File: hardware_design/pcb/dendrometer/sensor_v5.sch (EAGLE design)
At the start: 27 parts, among them J1 AVR_SPI_PRG_6PTH, Q2 MOSFET-P, U1 ATMEGA328P, U2 LM4040A20IDBZT

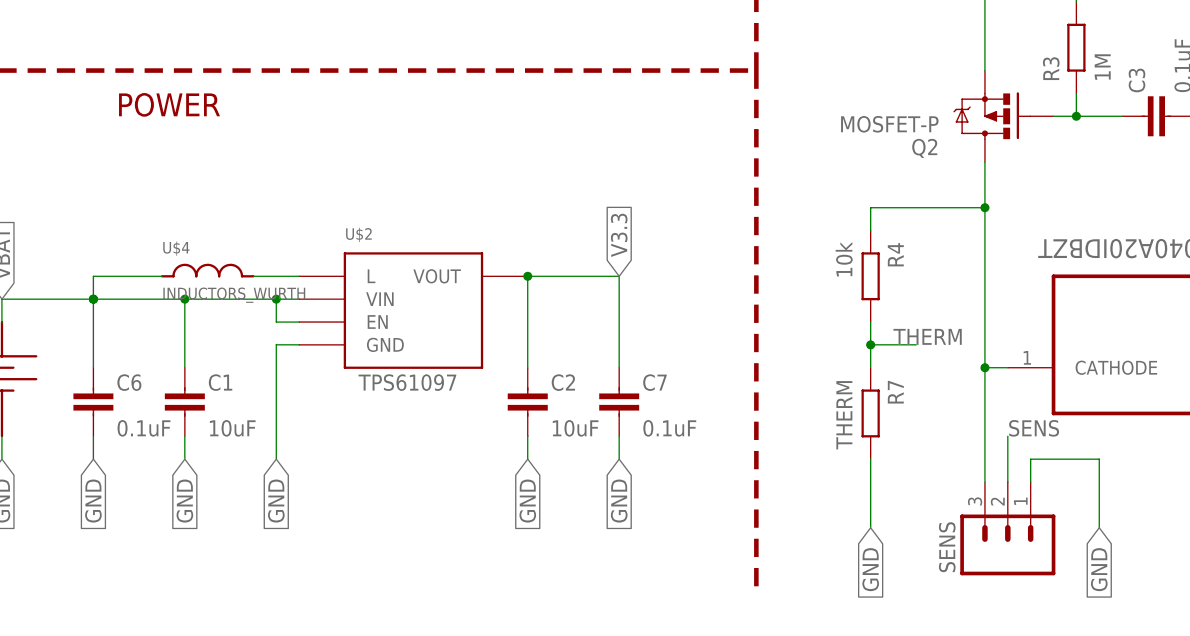
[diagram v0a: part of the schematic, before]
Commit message: cleanup..
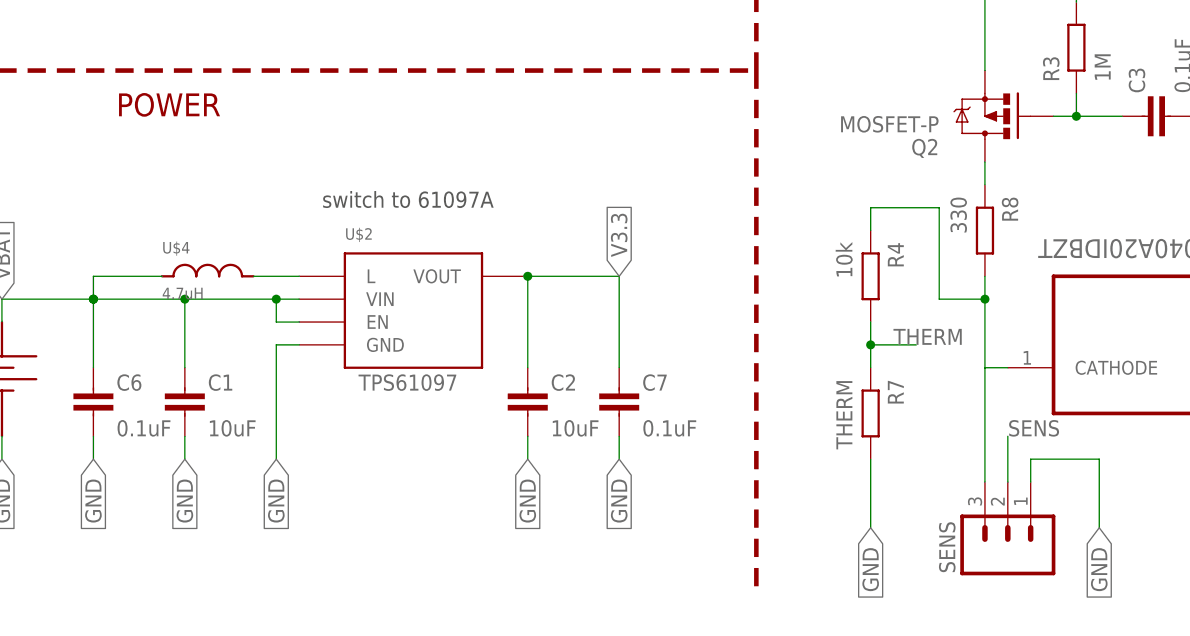
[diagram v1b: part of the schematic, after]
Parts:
- added R8: 330, passives-7351:RESISTOR0603-N
- U$4: value INDUCTORS_WURTH -> 4.7uH
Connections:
- new net S_EN: Q2.D, R8.P$1
- net V_REF: now also R8.P$2; no longer Q2.D
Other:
- note added: "switch to 61097A"
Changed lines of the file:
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@@
 <?xml version="1.0" encoding="utf-8"?>
 <!DOCTYPE eagle SYSTEM "eagle.dtd">
-<eagle version="7.2.0">
+<eagle version="7.6.0">
 <drawing>
 <settings>
@@
 <setting verticaltext="up"/>
 </settings>
-<grid distance="0.1" unitdist="inch" unit="inch" style="lines" multiple="1" display="no" altdistance="0.01" altunitdist="inch" altunit="inch"/>
+<grid distance="0.1" unitdist="inch" unit="inch" style="lines" multiple="1" display="yes" altdistance="0.01" altunitdist="inch" altunit="inch"/>
 <layers>
 <layer number="1" name="Top" color="4" fill="1" visible="no" active="no"/>
+<layer number="2" name="Route2" color="1" fill="3" visible="no" active="no"/>
+<layer number="3" name="Route3" color="4" fill="3" visible="no" active="no"/>
+<layer number="4" name="Route4" color="1" fill="4" visible="no" active="no"/>
+<layer number="5" name="Route5" color="4" fill="4" visible="no" active="no"/>
+<layer number="6" name="Route6" color="1" fill="8" visible="no" active="no"/>
+<layer number="7" name="Route7" color="4" fill="8" visible="no" active="no"/>
+<layer number="8" name="Route8" color="1" fill="2" visible="no" active="no"/>
+<layer number="9" name="Route9" color="4" fill="2" visible="no" active="no"/>
+<layer number="10" name="Route10" color="1" fill="7" visible="no" active="no"/>
+<layer number="11" name="Route11" color="4" fill="7" visible="no" active="no"/>
+<layer number="12" name="Route12" color="1" fill="5" visible="no" active="no"/>
+<layer number="13" name="Route13" color="4" fill="5" visible="no" active="no"/>
+<layer number="14" name="Route14" color="1" fill="6" visible="no" active="no"/>
+<layer number="15" name="Route15" color="4" fill="6" visible="no" active="no"/>
 <layer number="16" name="Bottom" color="1" fill="1" visible="no" active="no"/>
 <layer number="17" name="Pads" color="2" fill="1" visible="no" active="no"/>
@@
 <part name="U$5" library="LowPowerLab" deviceset="RFM69" device=""/>
 <part name="U$2" library="_my-parts" deviceset="TPS61097-33" device=""/>
-<part name="U$4" library="_my-parts" deviceset="INDUCTORS" device="_WURTH"/>
+<part name="U$4" library="_my-parts" deviceset="INDUCTORS" device="_WURTH" value="4.7uH"/>
 <part name="C1" library="passives-7351" deviceset="CAPACITOR" device="0805-N" value="10uF"/>
 <part name="C2" library="passives-7351" deviceset="CAPACITOR" device="0805-N" value="10uF"/>
@@
 <part name="R4" library="passives-7351" deviceset="RESISTOR" device="0603-N" value="10k"/>
 <part name="FRAME1" library="SparkFun-Aesthetics" deviceset="FRAME-A4L" device=""/>
+<part name="R8" library="passives-7351" deviceset="RESISTOR" device="0603-N" value="330"/>
 </parts>
 <sheets>
@@
 <text x="218.44" y="93.98" size="1.778" layer="94">ADC</text>
 <text x="129.54" y="93.98" size="1.778" layer="94">V_REF</text>
+<text x="50.8" y="48.26" size="1.778" layer="97">switch to 61097A</text>
 </plain>
 <instances>
@@
 <instance part="R4" gate="G$1" x="111.76" y="40.64" rot="R270"/>
 <instance part="FRAME1" gate="G$1" x="3.81" y="3.81"/>
+<instance part="R8" gate="G$1" x="124.46" y="45.72" rot="R270"/>
 </instances>
 <busses>
@@
 </segment>
 </net>
-<net name="V_REF" class="0">
-<segment>
-<pinref part="SENS" gate="J$1" pin="3"/>
-<wire x1="124.46" y1="17.78" x2="124.46" y2="30.48" width="0.1524" layer="91"/>
-<pinref part="U2" gate="A" pin="CATHODE"/>
-<wire x1="127" y1="30.48" x2="124.46" y2="30.48" width="0.1524" layer="91"/>
+<net name="S_EN" class="0">
+<segment>
+<pinref part="R8" gate="G$1" pin="P$1"/>
 <pinref part="Q2" gate="G$1" pin="D"/>
-<wire x1="124.46" y1="30.48" x2="124.46" y2="48.26" width="0.1524" layer="91"/>
-<junction x="124.46" y="30.48"/>
-<wire x1="124.46" y1="48.26" x2="124.46" y2="53.34" width="0.1524" layer="91"/>
-<pinref part="R4" gate="G$1" pin="P$1"/>
-<wire x1="111.76" y1="45.72" x2="111.76" y2="48.26" width="0.1524" layer="91"/>
-<wire x1="111.76" y1="48.26" x2="124.46" y2="48.26" width="0.1524" layer="91"/>
-<junction x="124.46" y="48.26"/>
+<wire x1="124.46" y1="50.8" x2="124.46" y2="53.34" width="0.1524" layer="91"/>
 </segment>
 </net>
@@
 </segment>
 </net>
+<net name="V_REF" class="0">
+<segment>
+<pinref part="U2" gate="A" pin="CATHODE"/>
+<wire x1="127" y1="30.48" x2="124.46" y2="30.48" width="0.1524" layer="91"/>
+<wire x1="124.46" y1="30.48" x2="124.46" y2="38.1" width="0.1524" layer="91"/>
+<pinref part="R8" gate="G$1" pin="P$2"/>
+<pinref part="SENS" gate="J$1" pin="3"/>
+<wire x1="124.46" y1="38.1" x2="124.46" y2="40.64" width="0.1524" layer="91"/>
+<wire x1="124.46" y1="30.48" x2="124.46" y2="17.78" width="0.1524" layer="91"/>
+<wire x1="124.46" y1="38.1" x2="119.38" y2="38.1" width="0.1524" layer="91"/>
+<junction x="124.46" y="38.1"/>
+<wire x1="119.38" y1="38.1" x2="119.38" y2="48.26" width="0.1524" layer="91"/>
+<pinref part="R4" gate="G$1" pin="P$1"/>
+<wire x1="111.76" y1="48.26" x2="111.76" y2="45.72" width="0.1524" layer="91"/>
+<wire x1="119.38" y1="48.26" x2="111.76" y2="48.26" width="0.1524" layer="91"/>
+</segment>
+</net>
